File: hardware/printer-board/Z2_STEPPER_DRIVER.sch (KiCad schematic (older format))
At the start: 9 parts, among them J11 MS_SELECT, J12 Z2, U7 A4988_MODULE

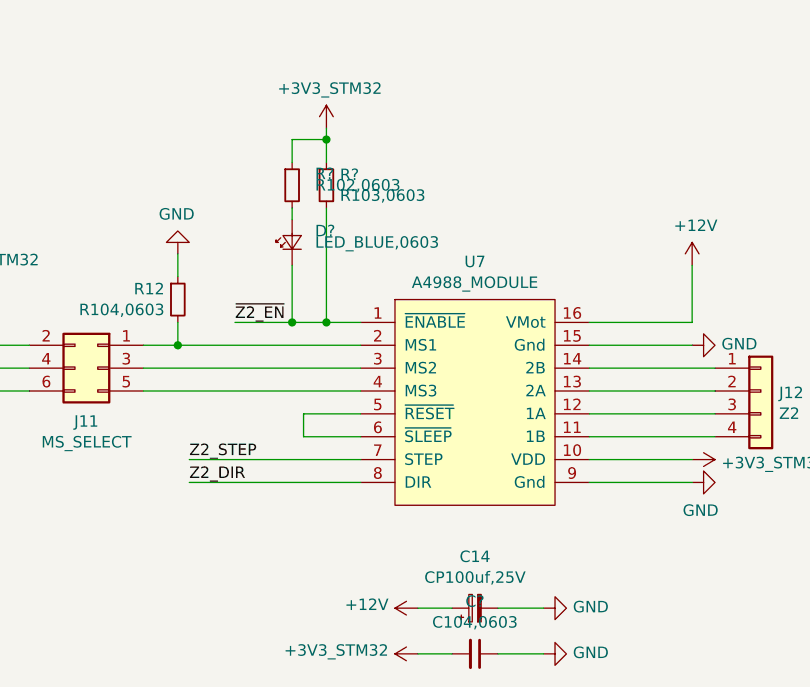
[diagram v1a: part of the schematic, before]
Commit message: update annotations,
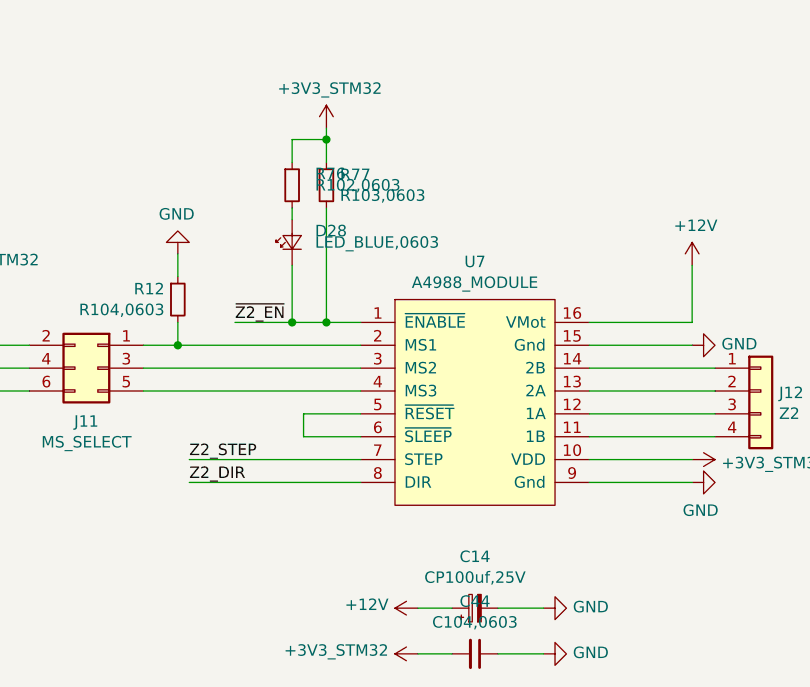
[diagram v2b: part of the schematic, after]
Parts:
- gave numbers to parts that had none: 4
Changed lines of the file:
@@
 $EndBitmap
 $Comp
-L taobao-components:+3V3_STM32 #PWR?
+L taobao-components:+3V3_STM32 #PWR091
 U 1 1 5CC40B53
 P 3500 2700
-F 0 "#PWR?" H 3500 2550 50  0001 C CNN
+F 0 "#PWR091" H 3500 2550 50  0001 C CNN
 F 1 "+3V3_STM32" H 3515 2873 50  0000 C CNN
 F 2 "" H 3500 2700 50  0001 C CNN
@@
 $EndComp
 $Comp
-L taobao-components:+3V3_STM32 #PWR?
+L taobao-components:+3V3_STM32 #PWR093
 U 1 1 5CC40B6A
 P 5400 4250
-F 0 "#PWR?" H 5400 4100 50  0001 C CNN
+F 0 "#PWR093" H 5400 4100 50  0001 C CNN
 F 1 "+3V3_STM32" V 5415 4378 50  0000 L CNN
 F 2 "" H 5400 4250 50  0001 C CNN
@@
 $EndComp
 $Comp
-L taobao-components:+3V3_STM32 #PWR?
+L taobao-components:+3V3_STM32 #PWR092
 U 1 1 5CC40B93
 P 6600 3400
-F 0 "#PWR?" H 6600 3250 50  0001 C CNN
+F 0 "#PWR092" H 6600 3250 50  0001 C CNN
 F 1 "+3V3_STM32" V 6615 3528 50  0000 L CNN
 F 2 "" H 6600 3400 50  0001 C CNN
@@
 $EndComp
 $Comp
-L taobao-c:C104,0603 C?
+L taobao-c:C104,0603 C44
 U 1 1 5CC40C89
 P 5650 4250
-F 0 "C?" V 5421 4250 50  0000 C CNN
+F 0 "C44" V 5421 4250 50  0000 C CNN
 F 1 "C104,0603" V 5512 4250 50  0000 C CNN
 F 2 "Capacitor_SMD:C_0603_1608Metric_Pad1.05x0.95mm_HandSolder" H 5650 4250 50  0001 C CNN
@@
 AR Path="/5CC0A53C/5CC5B1C2" Ref="R?"  Part="1"
 AR Path="/5CC0A8C5/5CC5B1C2" Ref="R?"  Part="1"
-AR Path="/5CC0A8CA/5CC5B1C2" Ref="R?"  Part="1"
+AR Path="/5CC0A8CA/5CC5B1C2" Ref="R77"  Part="1"
 AR Path="/5CC0A8CF/5CC5B1C2" Ref="R?"  Part="1"
 AR Path="/5CC0AEC9/5CC5B1C2" Ref="R?"  Part="1"
-F 0 "R?" H 5059 2246 50  0000 L CNN
+F 0 "R77" H 5059 2246 50  0000 L CNN
 F 1 "R103,0603" H 5059 2155 50  0000 L CNN
 F 2 "Resistor_SMD:R_0603_1608Metric_Pad1.05x0.95mm_HandSolder" H 5000 2200 50  0001 C CNN
@@
 P 5000 1950
 AR Path="/5CC0AEC9/5CC5B1CA" Ref="#PWR?"  Part="1"
-AR Path="/5CC0A8CA/5CC5B1CA" Ref="#PWR?"  Part="1"
-F 0 "#PWR?" H 5000 1800 50  0001 C CNN
+AR Path="/5CC0A8CA/5CC5B1CA" Ref="#PWR090"  Part="1"
+F 0 "#PWR090" H 5000 1800 50  0001 C CNN
 F 1 "+3V3_STM32" H 5015 2123 50  0000 C CNN
 F 2 "" H 5000 1950 50  0001 C CNN
@@
 AR Path="/5CC15C35/5CC5B1D0" Ref="R?"  Part="1"
 AR Path="/5CC0AEC9/5CC5B1D0" Ref="R?"  Part="1"
-AR Path="/5CC0A8CA/5CC5B1D0" Ref="R?"  Part="1"
-F 0 "R?" H 4950 2250 50  0000 L CNN
+AR Path="/5CC0A8CA/5CC5B1D0" Ref="R76"  Part="1"
+F 0 "R76" H 4950 2250 50  0000 L CNN
 F 1 "R102,0603" H 4950 2200 50  0000 L CNN
 F 2 "Resistor_SMD:R_0603_1608Metric_Pad1.05x0.95mm_HandSolder" H 4850 2200 50  0001 C CNN
@@
 AR Path="/5CC15C35/5CC5B1D7" Ref="D?"  Part="1"
 AR Path="/5CC0AEC9/5CC5B1D7" Ref="D?"  Part="1"
-AR Path="/5CC0A8CA/5CC5B1D7" Ref="D?"  Part="1"
-F 0 "D?" V 4900 2350 50  0000 R CNN
+AR Path="/5CC0A8CA/5CC5B1D7" Ref="D28"  Part="1"
+F 0 "D28" V 4900 2350 50  0000 R CNN
 F 1 "LED_BLUE,0603" V 4850 2350 50  0000 R CNN
 F 2 "LED_SMD:LED_0603_1608Metric_Pad1.05x0.95mm_HandSolder" V 4850 2450 50  0001 C CNN

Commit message: update,
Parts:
- J12: footprint Connector_PinHeader_2.00mm:PinHeader_1x04_P2.00mm_Vertical -> footprint-lib:b4b-ph-kl,stepper_terminal
- U7: footprint Module:Pololu_Breakout-16_15.2x20.3mm -> footprint-lib:Pololu_Breakout-16_15.2x20.3mm
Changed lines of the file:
@@
 F 0 "U7" H 5650 3765 50  0000 C CNN
 F 1 "A4988_MODULE" H 5650 3674 50  0000 C CNN
-F 2 "Module:Pololu_Breakout-16_15.2x20.3mm" H 5650 3200 50  0001 C CNN
+F 2 "footprint-lib:Pololu_Breakout-16_15.2x20.3mm" H 5650 3200 50  0001 C CNN
 F 3 "" H 5650 3200 50  0001 C CNN
 	1    5650 3150
@@
 F 0 "J12" H 6980 3092 50  0000 L CNN
 F 1 "Z2" H 6980 3001 50  0000 L CNN
-F 2 "Connector_PinHeader_2.00mm:PinHeader_1x04_P2.00mm_Vertical" H 6900 3100 50  0001 C CNN
+F 2 "footprint-lib:b4b-ph-kl,stepper_terminal" H 6900 3100 50  0001 C CNN
 F 3 "~" H 6900 3100 50  0001 C CNN
 	1    6900 3100
